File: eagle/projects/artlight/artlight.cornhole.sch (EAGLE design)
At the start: 28 parts, among them T1 2N2222, T2 2N2222, T3 2N2222, T4 2N2222, T5 2N2222, T6 2N2222, T7 2N2222, T8 2N2222, T9 2N2222

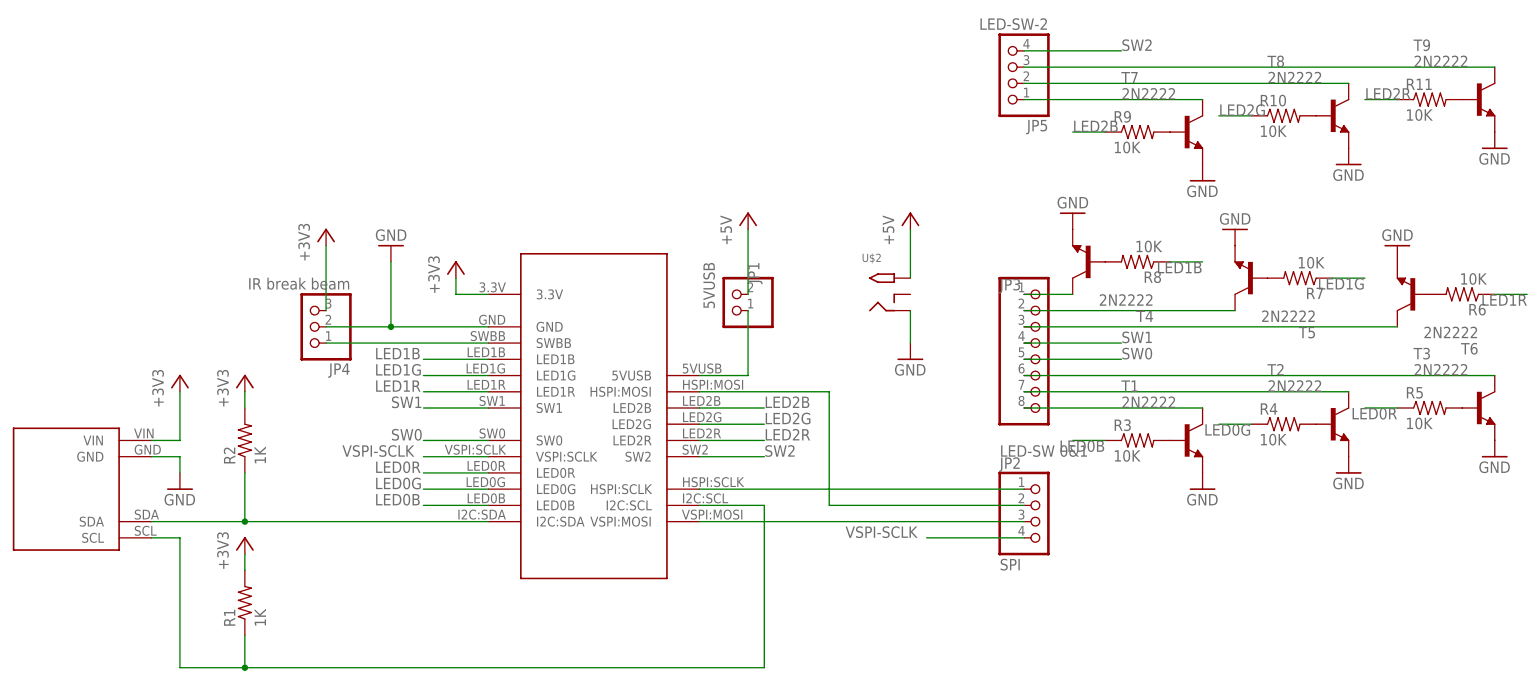
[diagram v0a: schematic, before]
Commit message: eagle: artlight.cornhole, pins
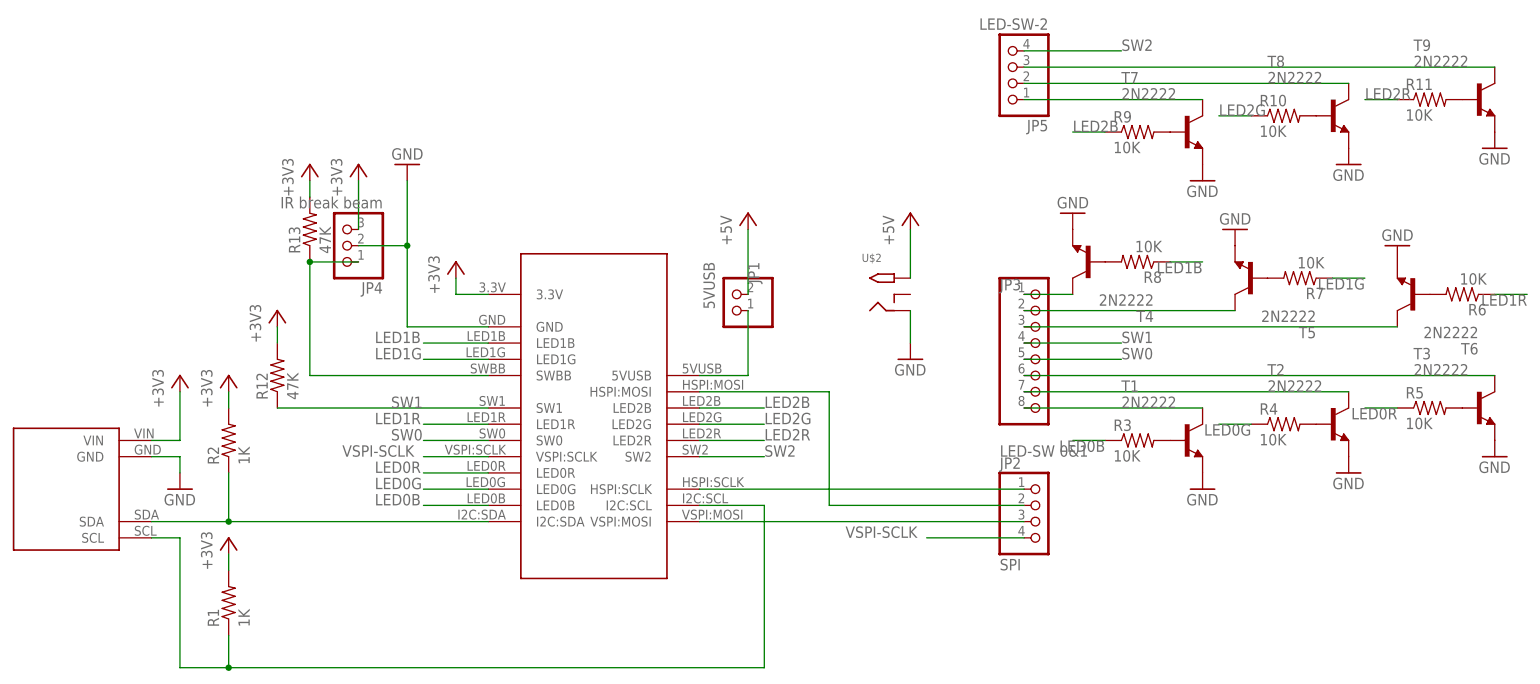
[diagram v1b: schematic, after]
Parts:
- added R12, R13: 47K, rcl:R-US_0204/7
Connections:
- net +3V3: now also R12.2, R13.2
- net SW1: now also R12.1
- net SWBB: now also R13.1
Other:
- moved on the sheet: JP4, R1, R2
